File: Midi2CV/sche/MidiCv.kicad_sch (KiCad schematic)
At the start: 9 parts, among them U1 STM32F103C8T6_BD, U2 6N138

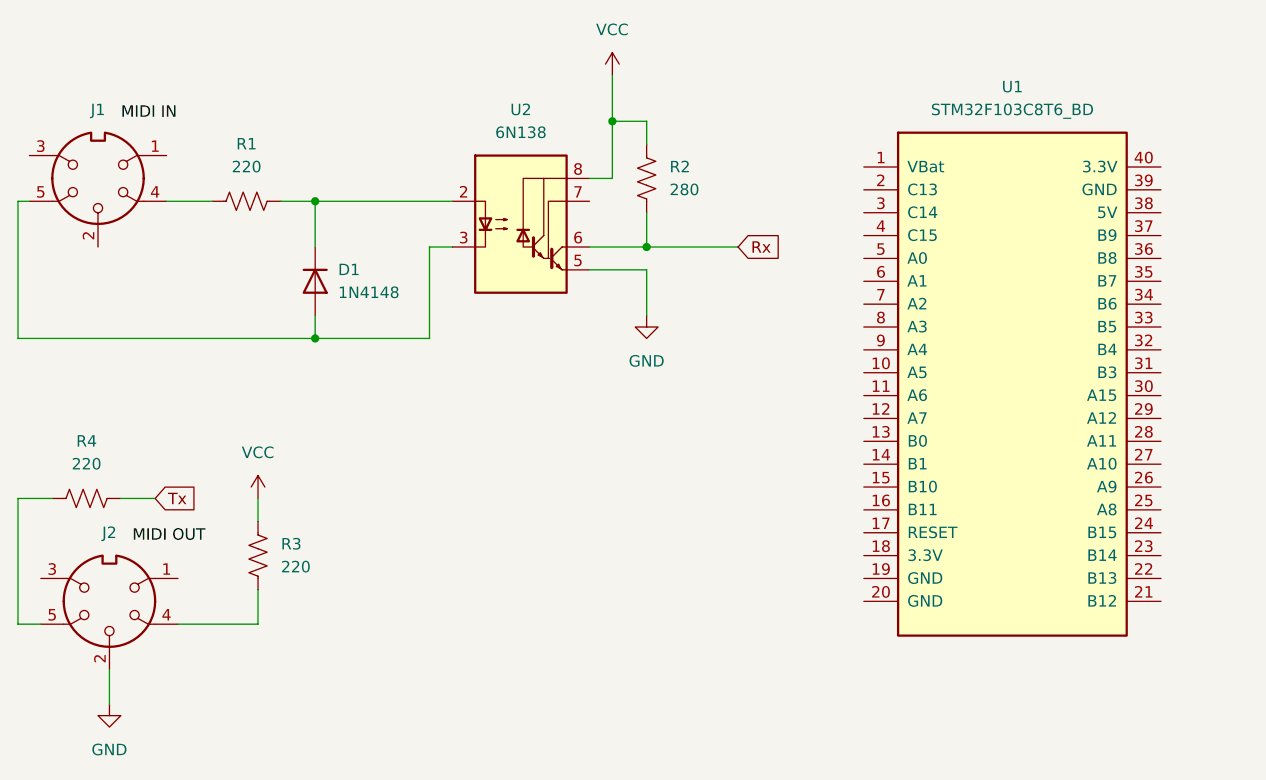
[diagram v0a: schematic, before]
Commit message: midi input print out v0.1
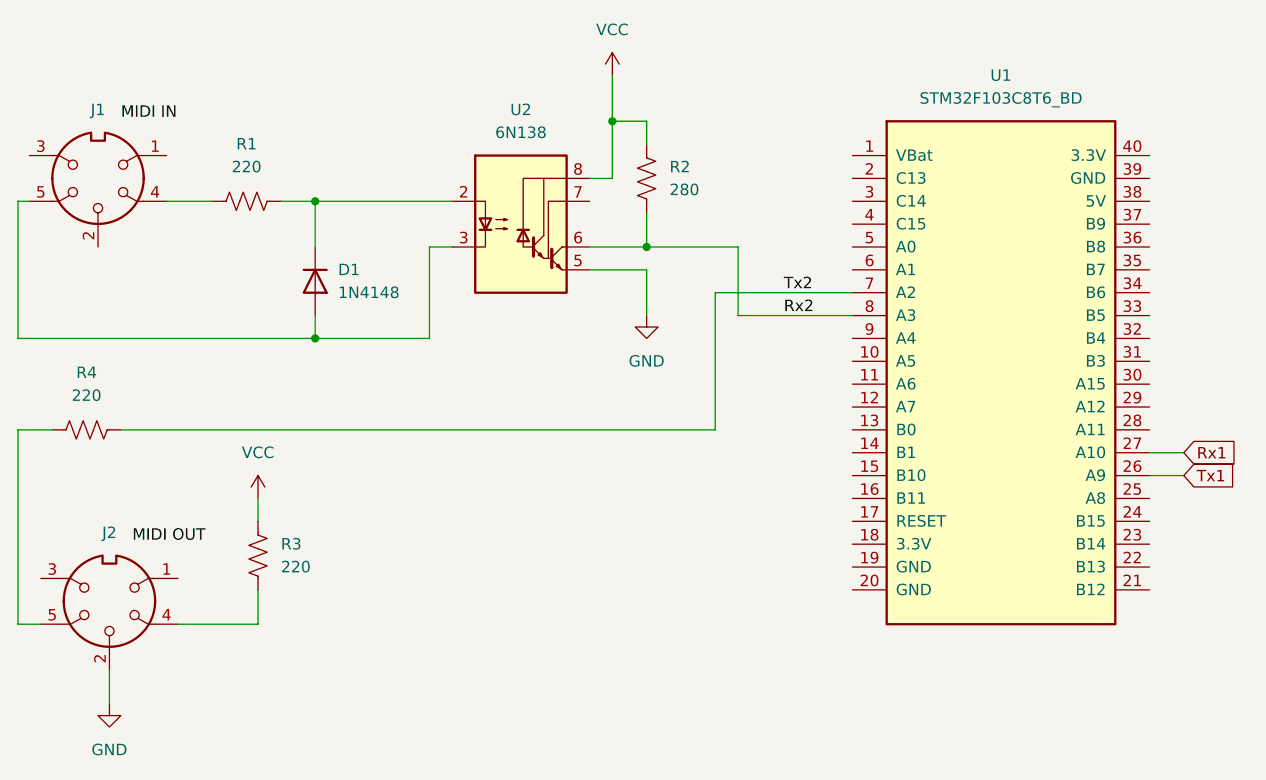
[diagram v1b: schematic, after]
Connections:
- net Rx is gone; now on net Rx2: R2.1, U2.6 (VO2)
- net Tx is gone; now on net Tx2: R4.1
- net Tx1: now reaches U1.26 (A9)
- net Rx1: now reaches U1.27 (A10)
- net Tx2: now reaches U1.7 (A2)
- net Rx2: now reaches U1.8 (A3)
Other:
- moved on the sheet: R4, U1
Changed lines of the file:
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@@
     (stroke (width 0) (type default))
   )
-  (wire (pts (xy 29.21 88.9) (xy 25.4 88.9))
+  (wire (pts (xy 151.13 86.36) (xy 154.94 86.36))
+    (stroke (width 0) (type default))
+  )
+  (wire (pts (xy 29.21 81.28) (xy 25.4 81.28))
     (stroke (width 0) (type default))
   )
@@
     (stroke (width 0) (type default))
   )
+  (wire (pts (xy 102.87 81.28) (xy 102.87 66.04))
+    (stroke (width 0) (type default))
+  )
   (wire (pts (xy 91.44 53.34) (xy 91.44 46.99))
     (stroke (width 0) (type default))
   )
+  (wire (pts (xy 151.13 83.82) (xy 154.94 83.82))
+    (stroke (width 0) (type default))
+  )
+  (wire (pts (xy 36.83 81.28) (xy 102.87 81.28))
+    (stroke (width 0) (type default))
+  )
   (wire (pts (xy 43.18 102.87) (xy 52.07 102.87))
     (stroke (width 0) (type default))
@@
     (stroke (width 0) (type default))
   )
-  (wire (pts (xy 36.83 88.9) (xy 40.64 88.9))
+  (wire (pts (xy 102.87 66.04) (xy 118.11 66.04))
     (stroke (width 0) (type default))
   )
@@
     (stroke (width 0) (type default))
   )
+  (wire (pts (xy 105.41 68.58) (xy 118.11 68.58))
+    (stroke (width 0) (type default))
+  )
   (wire (pts (xy 26.67 55.88) (xy 25.4 55.88))
     (stroke (width 0) (type default))
@@
     (stroke (width 0) (type default))
   )
+  (wire (pts (xy 105.41 68.58) (xy 105.41 60.96))
+    (stroke (width 0) (type default))
+  )
   (wire (pts (xy 88.9 63.5) (xy 95.25 63.5))
     (stroke (width 0) (type default))
@@
     (stroke (width 0) (type default))
   )
-  (wire (pts (xy 25.4 88.9) (xy 25.4 102.87))
+  (wire (pts (xy 25.4 81.28) (xy 25.4 102.87))
     (stroke (width 0) (type default))
   )
@@
     (effects (font (size 1.27 1.27)) (justify left bottom))
   )
+  (label "Tx2" (at 110.49 66.04 0) (fields_autoplaced)
+    (effects (font (size 1.27 1.27)) (justify left bottom))
+  )
   (label "MIDI OUT" (at 38.1 93.98 0) (fields_autoplaced)
     (effects (font (size 1.27 1.27)) (justify left bottom))
   )
-  (global_label "Rx" (shape input) (at 105.41 60.96 0) (fields_autoplaced)
+  (label "Rx2" (at 110.49 68.58 0) (fields_autoplaced)
+    (effects (font (size 1.27 1.27)) (justify left bottom))
+  )
+  (global_label "Tx1" (shape input) (at 154.94 86.36 0) (fields_autoplaced)
     (effects (font (size 1.27 1.27)) (justify left))
-    (property "Intersheetrefs" "${INTERSHEET_REFS}" (at 110.6933 60.96 0)
+    (property "Intersheetrefs" "${INTERSHEET_REFS}" (at 161.1304 86.36 0)
       (effects (font (size 1.27 1.27)) (justify left) hide)
     )
   )
-  (global_label "Tx" (shape input) (at 40.64 88.9 0) (fields_autoplaced)
+  (global_label "Rx1" (shape input) (at 154.94 83.82 0) (fields_autoplaced)
     (effects (font (size 1.27 1.27)) (justify left))
-    (property "Intersheetrefs" "${INTERSHEET_REFS}" (at 45.6209 88.9 0)
+    (property "Intersheetrefs" "${INTERSHEET_REFS}" (at 161.4328 83.82 0)
       (effects (font (size 1.27 1.27)) (justify left) hide)
     )
@@
     )
   )
-  (symbol (lib_id "RetroElec:STM32F103C8T6_BD") (at 135.89 76.2 0) (unit 1)
-    (in_bom yes) (on_board yes) (dnp no) (fields_autoplaced)
-    (property "Reference" "U1" (at 135.89 43.18 0)
-      (effects (font (size 1.27 1.27)))
-    )
-    (property "Value" "STM32F103C8T6_BD" (at 135.89 45.72 0)
-      (effects (font (size 1.27 1.27)))
-    )
-    (property "Footprint" "" (at 135.89 72.39 0)
-      (effects (font (size 1.27 1.27)) hide)
-    )
-    (property "Datasheet" "" (at 138.43 106.68 0)
+  (symbol (lib_id "RetroElec:STM32F103C8T6_BD") (at 134.62 74.93 0) (unit 1)
+    (in_bom yes) (on_board yes) (dnp no) (fields_autoplaced)
+    (property "Reference" "U1" (at 134.62 41.91 0)
+      (effects (font (size 1.27 1.27)))
+    )
+    (property "Value" "STM32F103C8T6_BD" (at 134.62 44.45 0)
+      (effects (font (size 1.27 1.27)))
+    )
+    (property "Footprint" "" (at 134.62 71.12 0)
+      (effects (font (size 1.27 1.27)) hide)
+    )
+    (property "Datasheet" "" (at 137.16 105.41 0)
       (effects (font (size 1.27 1.27)) hide)
     )
@@
     )
   )
-  (symbol (lib_id "Device:R_US") (at 33.02 88.9 270) (unit 1)
-    (in_bom yes) (on_board yes) (dnp no) (fields_autoplaced)
-    (property "Reference" "R4" (at 33.02 82.55 90)
-      (effects (font (size 1.27 1.27)))
-    )
-    (property "Value" "220" (at 33.02 85.09 90)
-      (effects (font (size 1.27 1.27)))
-    )
-    (property "Footprint" "" (at 32.766 89.916 90)
-      (effects (font (size 1.27 1.27)) hide)
-    )
-    (property "Datasheet" "~" (at 33.02 88.9 0)
-      (effects (font (size 1.27 1.27)) hide)
-    )
+  (symbol (lib_id "Device:R_US") (at 33.02 81.28 270) (unit 1)
+    (in_bom yes) (on_board yes) (dnp no) (fields_autoplaced)
+    (property "Reference" "R4" (at 33.02 74.93 90)
+      (effects (font (size 1.27 1.27)))
+    )
+    (property "Value" "220" (at 33.02 77.47 90)
+      (effects (font (size 1.27 1.27)))
+    )
+    (property "Footprint" "" (at 32.766 82.296 90)
+      (effects (font (size 1.27 1.27)) hide)
+    )
+    (property "Datasheet" "~" (at 33.02 81.28 0)
+      (effects (font (size 1.27 1.27)) hide)
+    )
